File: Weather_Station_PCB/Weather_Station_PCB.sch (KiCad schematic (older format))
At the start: 3 parts

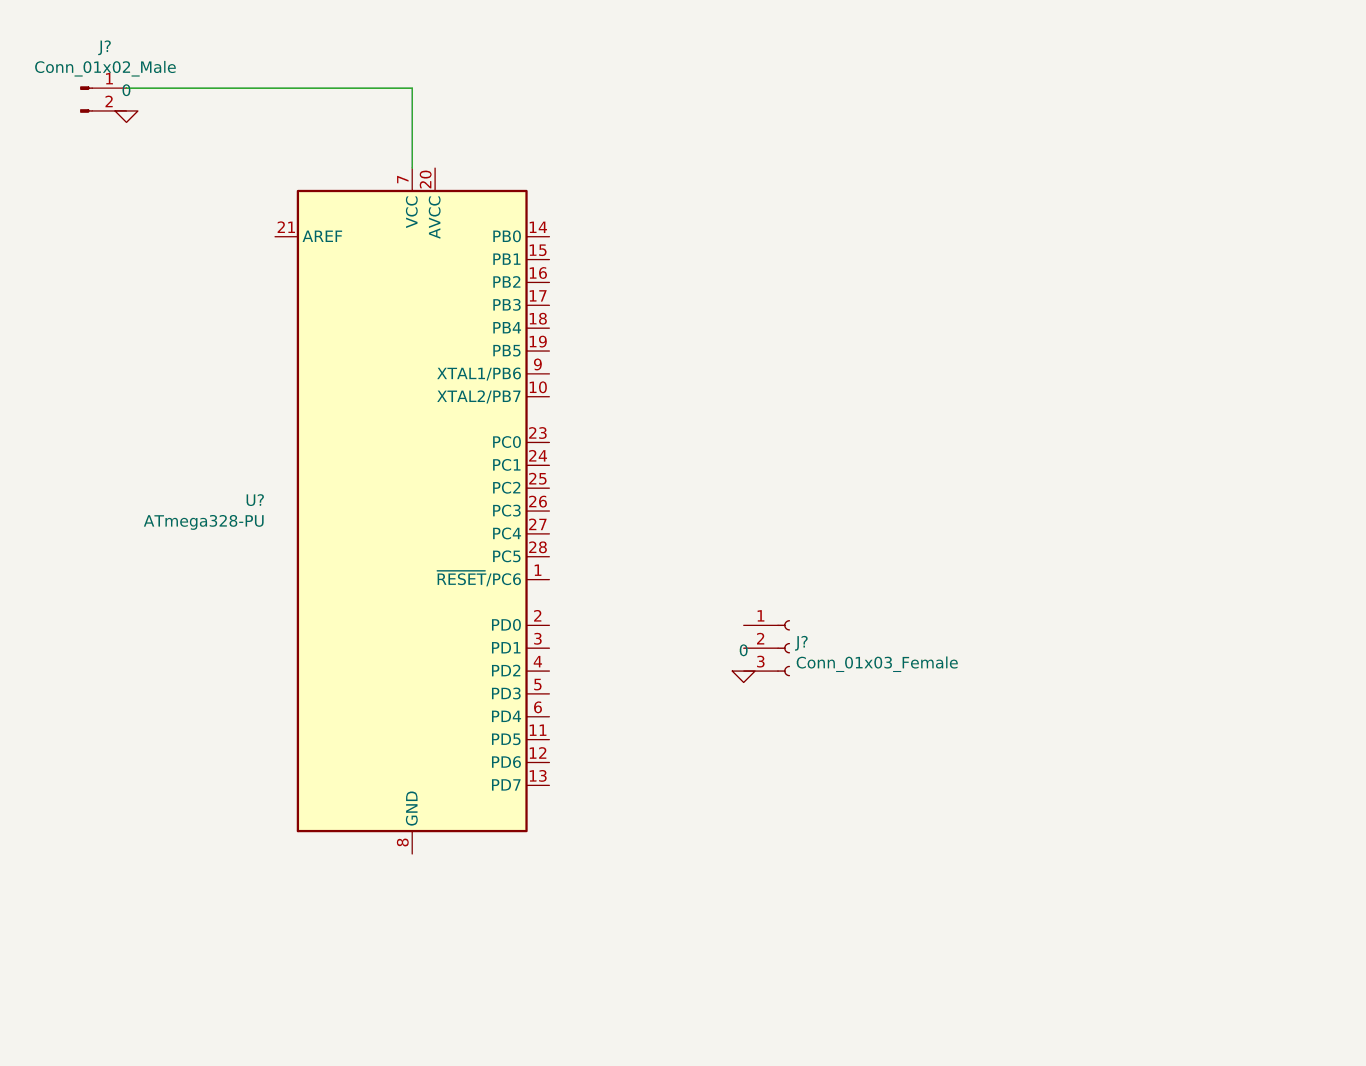
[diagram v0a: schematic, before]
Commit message: Adding the stuff I have worked on, big update
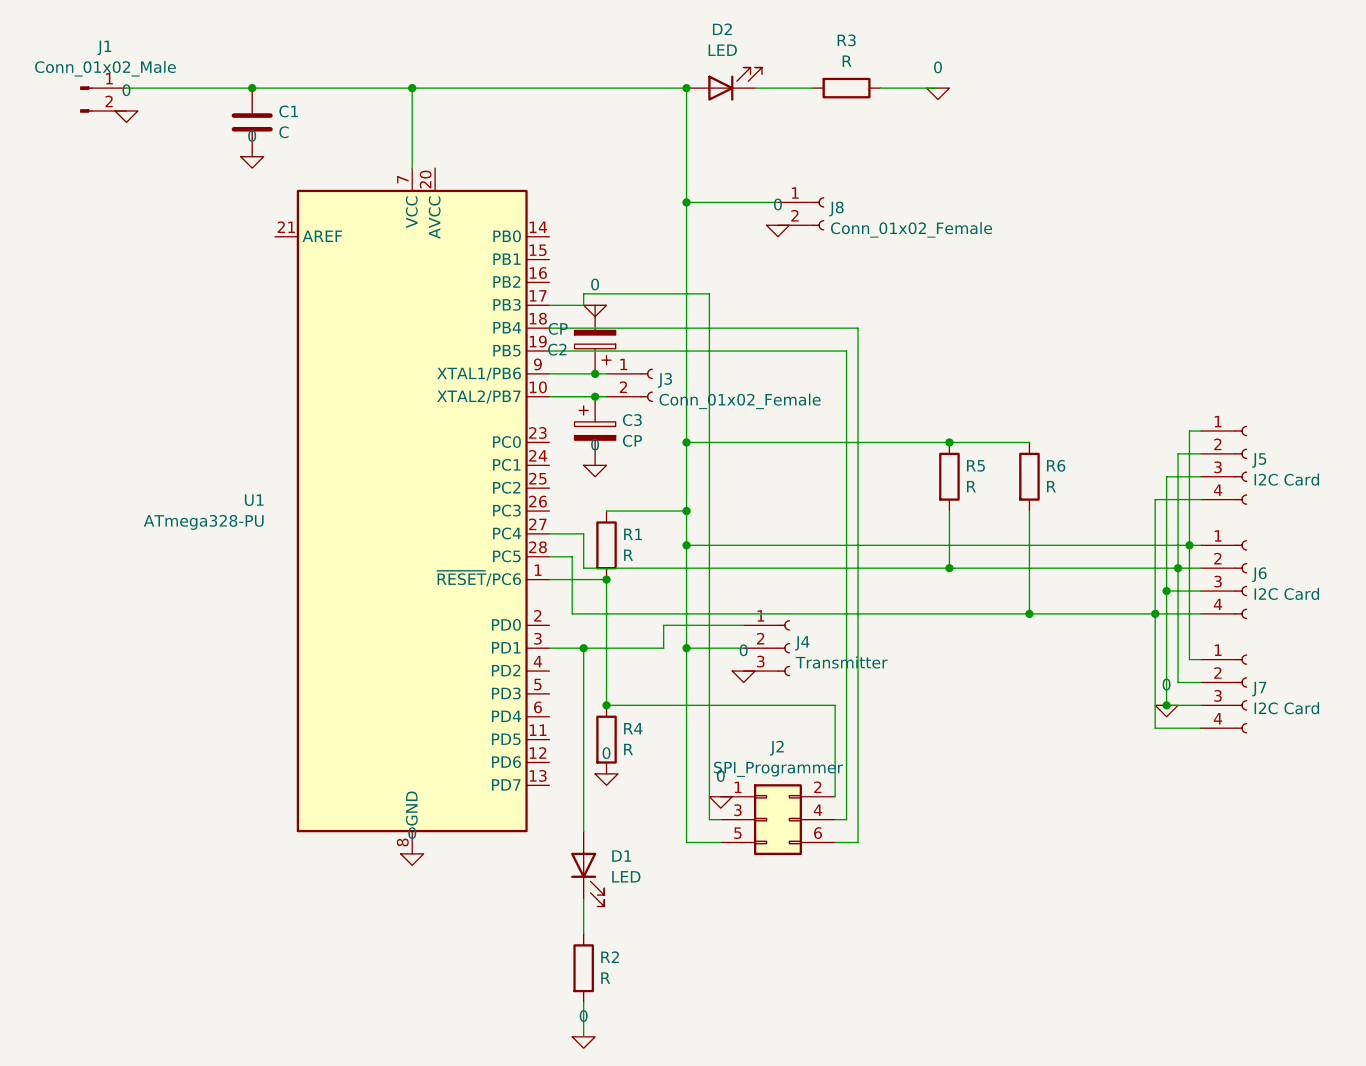
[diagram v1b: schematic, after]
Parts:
- added C1: C, Capacitor_THT:CP_Radial_D5.0mm_P2.50mm, symbol Device:C
- added C2, C3: CP, Capacitor_SMD:C_1206_3216Metric, symbol Device:CP
- added D1, D2: LED, LED_SMD:LED_1206_3216Metric, symbol Device:LED
- added J2: SPI_Programmer, Connector_PinHeader_2.54mm:PinHeader_2x03_P2.54mm_Vertical, symbol Connector_Generic:Conn_02x03_Odd_Even
- added J3: Conn_01x02_Female, Crystal:Crystal_HC49-4H_Vertical, symbol Connector:Conn_01x02_Female
- added J5, J6, J7: I2C Card, Connector_PinSocket_2.54mm:PinSocket_1x04_P2.54mm_Vertical, symbol Connector:Conn_01x04_Female
- added J8: Conn_01x02_Female, TerminalBlock_Phoenix:TerminalBlock_Phoenix_PT-1,5-2-3.5-H_1x02_P3.50mm_Horizontal, symbol Connector:Conn_01x02_Female
- added R1, R2, R3, R4, R5, R6: R, Resistor_SMD:R_1206_3216Metric, symbol Device:R
- J1: renamed from J?; footprint (none) -> Connector_PinSocket_2.54mm:PinSocket_1x02_P2.54mm_Vertical
- J4: renamed from J?; value Conn_01x03_Female -> Transmitter; footprint (none) -> Connector_PinSocket_2.54mm:PinSocket_1x03_P2.54mm_Vertical
- gave numbers to parts that had none: 1
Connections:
- net 0: now also U1.22 (GND), U1.8 (GND), C1.2, C2.2, C3.2, J2.1 (Pin_1), J5.3 (Pin_3), J6.3 (Pin_3), J7.3 (Pin_3), J8.2 (Pin_2), R2.2, R3.1, R4.2
- net at U1.1 (~RESET~/PC6): now also J2.2 (Pin_2), R1.2, R4.1
- net at U1.10 (XTAL2/PB7): now also C3.1, J3.2 (Pin_2)
- net at U1.17 (PB3): now also J2.3 (Pin_3)
- net at U1.18 (PB4): now also J2.6 (Pin_6)
- net at U1.19 (PB5): now also J2.4 (Pin_4)
- net at U1.27 (PC4): now also J5.2 (Pin_2), J6.2 (Pin_2), J7.2 (Pin_2), R5.2
- net at U1.28 (PC5): now also J5.4 (Pin_4), J6.4 (Pin_4), J7.4 (Pin_4), R6.2
- net at U1.3 (PD1): now also J4.1 (Pin_1), D1.2 (A)
- net at J1.1 (Pin_1), U1.7 (VCC): now also J4.2 (Pin_2), C1.1, D2.2 (A), J2.5 (Pin_5), J5.1 (Pin_1), J6.1 (Pin_1), J7.1 (Pin_1), J8.1 (Pin_1), R1.1, R5.1, R6.1
- net at U1.9 (XTAL1/PB6): now also C2.1, J3.1 (Pin_1)
- new net: D2.1 (K), R3.2
- new net: D1.1 (K), R2.1
